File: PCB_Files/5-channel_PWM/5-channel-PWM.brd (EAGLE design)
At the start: 58 x 63 mm, 28 parts, among them Q1 N-MOS, Q2 N-MOS, Q3 N-MOS, Q4 N-MOS, Q5 N-MOS

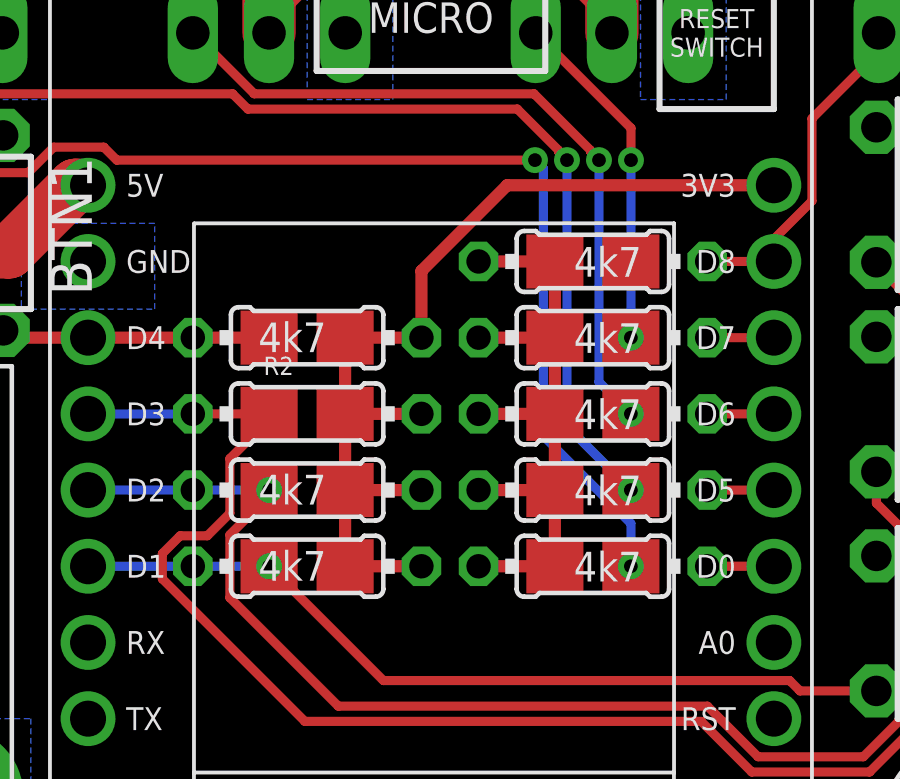
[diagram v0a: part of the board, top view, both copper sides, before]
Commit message: fixed design
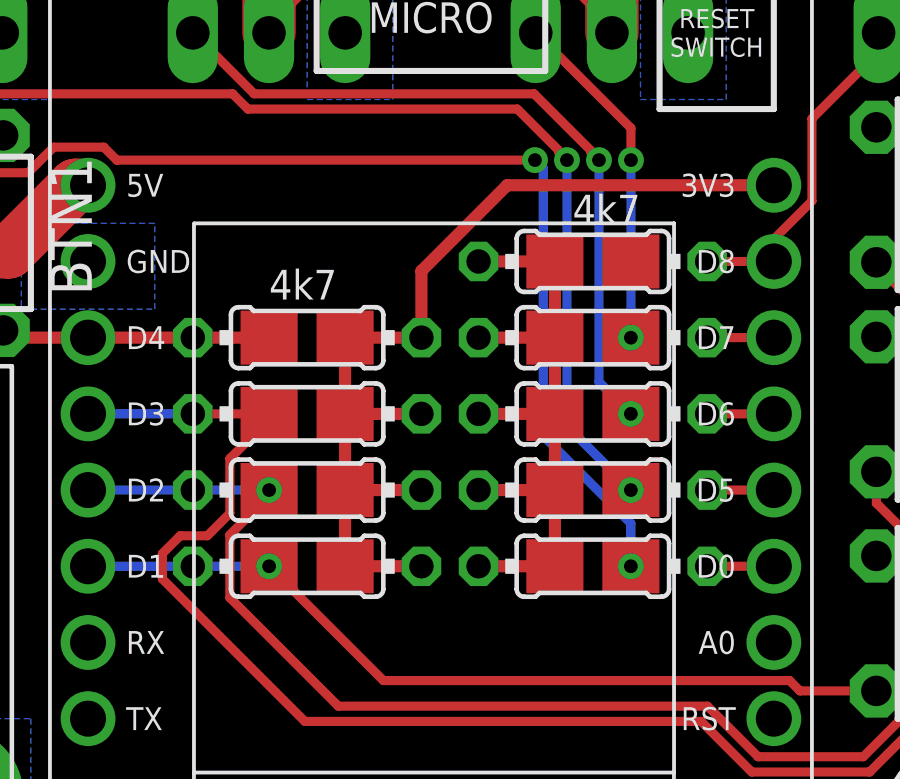
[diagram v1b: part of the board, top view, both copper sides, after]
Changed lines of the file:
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@@
 <setting verticaltext="up"/>
 </settings>
-<grid distance="1" unitdist="mm" unit="mm" style="lines" multiple="1" display="yes" altdistance="1" altunitdist="mm" altunit="mm"/>
+<grid distance="12.5" unitdist="mil" unit="mil" style="lines" multiple="1" display="yes" altdistance="1" altunitdist="mm" altunit="mm"/>
 <layers>
 <layer number="1" name="Top" color="4" fill="1" visible="yes" active="yes"/>
@@
 </element>
 <element name="R1" library="diyHue" package="MULTI_RESISTOR" value="4k7" x="30.48" y="21.59" smashed="yes">
-<attribute name="VALUE" x="28.8544" y="21.1074" size="0.9906" layer="21" ratio="10"/>
+<attribute name="VALUE" x="29.21" y="22.86" size="0.9906" layer="21" ratio="10"/>
 </element>
 <element name="H1" library="holes" package="3,0-PAD" value="MOUNT-PAD-ROUND3.0" x="5" y="5"/>
@@
 <element name="H4" library="holes" package="3,0-PAD" value="MOUNT-PAD-ROUND3.0" x="5" y="58"/>
 <element name="BTN3" library="schalter_taster" package="KSM611A" value="" x="52.705" y="19.3675" rot="R180"/>
-<element name="R4" library="diyHue" package="MULTI_RESISTOR" value="4k7" x="30.48" y="16.51" smashed="yes">
-<attribute name="VALUE" x="28.8544" y="16.0274" size="0.9906" layer="21" ratio="10"/>
-</element>
+<element name="R4" library="diyHue" package="MULTI_RESISTOR" value="4k7" x="30.48" y="16.51" smashed="yes"/>
 <element name="Q1" library="transistor-fet" package="TO220" value="N-MOS" x="6.35" y="38.1"/>
 <element name="Q2" library="transistor-fet" package="TO220" value="N-MOS" x="17.78" y="38.1"/>
@@
 <attribute name="VALUE" x="16.5576" y="54.0258" size="1.27" layer="27" ratio="10"/>
 </element>
-<element name="R3" library="diyHue" package="MULTI_RESISTOR" value="4k7" x="40.005" y="13.97" smashed="yes" rot="R180">
-<attribute name="VALUE" x="41.6306" y="14.4526" size="0.9906" layer="21" ratio="10" rot="R180"/>
-</element>
-<element name="R6" library="diyHue" package="MULTI_RESISTOR" value="4k7" x="40.005" y="16.51" smashed="yes" rot="R180">
-<attribute name="VALUE" x="41.6306" y="16.9926" size="0.9906" layer="21" ratio="10" rot="R180"/>
-</element>
-<element name="R7" library="diyHue" package="MULTI_RESISTOR" value="4k7" x="40.005" y="19.05" smashed="yes" rot="R180">
-<attribute name="VALUE" x="41.6306" y="19.5326" size="0.9906" layer="21" ratio="10" rot="R180"/>
-</element>
-<element name="R8" library="diyHue" package="MULTI_RESISTOR" value="4k7" x="40.005" y="21.59" smashed="yes" rot="R180">
-<attribute name="VALUE" x="41.6306" y="22.0726" size="0.9906" layer="21" ratio="10" rot="R180"/>
-</element>
+<element name="R3" library="diyHue" package="MULTI_RESISTOR" value="4k7" x="40.005" y="13.97" smashed="yes" rot="R180"/>
+<element name="R6" library="diyHue" package="MULTI_RESISTOR" value="4k7" x="40.005" y="16.51" smashed="yes" rot="R180"/>
+<element name="R7" library="diyHue" package="MULTI_RESISTOR" value="4k7" x="40.005" y="19.05" smashed="yes" rot="R180"/>
+<element name="R8" library="diyHue" package="MULTI_RESISTOR" value="4k7" x="40.005" y="21.59" smashed="yes" rot="R180"/>
 <element name="R9" library="diyHue" package="MULTI_RESISTOR" value="4k7" x="40.005" y="24.13" smashed="yes" rot="R180">
-<attribute name="VALUE" x="41.6306" y="24.6126" size="0.9906" layer="21" ratio="10" rot="R180"/>
+<attribute name="VALUE" x="41.5925" y="26.3525" size="0.9906" layer="21" ratio="10" rot="R180"/>
 </element>
 <element name="BTN4" library="schalter_taster" package="KSM611A" value="" x="52.705" y="12.065" rot="R180"/>
-<element name="R5" library="diyHue" package="MULTI_RESISTOR" value="4k7" x="30.48" y="13.97" smashed="yes">
-<attribute name="VALUE" x="28.8544" y="13.4874" size="0.9906" layer="21" ratio="10"/>
-</element>
+<element name="R5" library="diyHue" package="MULTI_RESISTOR" value="4k7" x="30.48" y="13.97" smashed="yes"/>
 <element name="JP1" library="pinhead-2" package="1X06-S" value="" x="29.21" y="60.96" smashed="yes">
 <attribute name="VALUE" x="21.59" y="57.785" size="1.27" layer="27"/>
@@
 <element name="U$1" library="diyHue" package="BUCK_CONVERTER_TE818" value="BUCK_CONVERTER_TE818" x="15.24" y="19.05" rot="R270"/>
 <element name="BTN2" library="schalter_taster" package="KSM611A" value="" x="52.705" y="26.3525" rot="R180"/>
-<element name="R2" library="diyHue" package="MULTI_RESISTOR" value="4k7" x="30.48" y="19.05"/>
+<element name="R2" library="diyHue" package="MULTI_RESISTOR" value="4k7" x="30.48" y="19.05" smashed="yes"/>
 </elements>
 <signals>
